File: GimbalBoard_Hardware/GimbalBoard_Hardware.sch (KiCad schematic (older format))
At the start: 5 parts

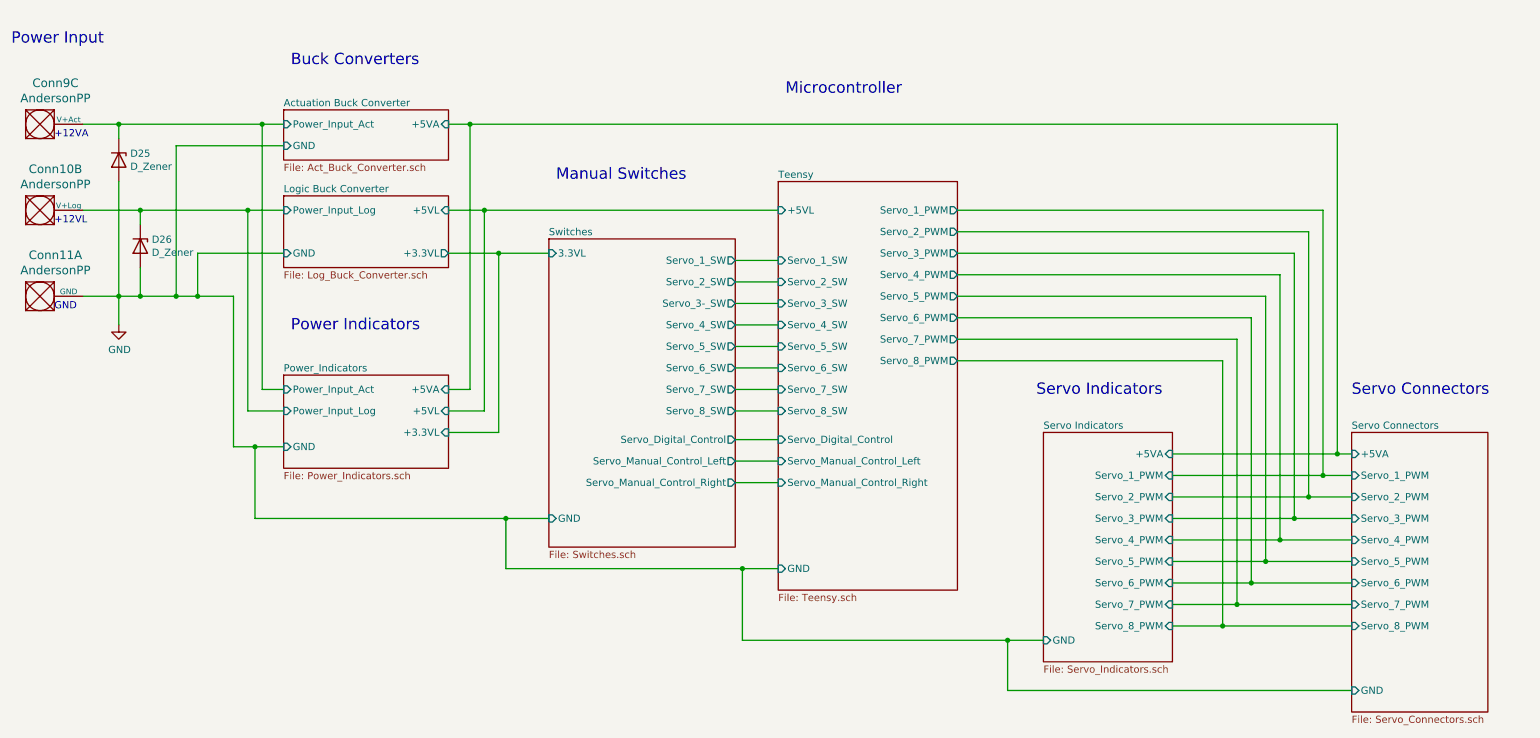
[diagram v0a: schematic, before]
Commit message: Post PDR changes
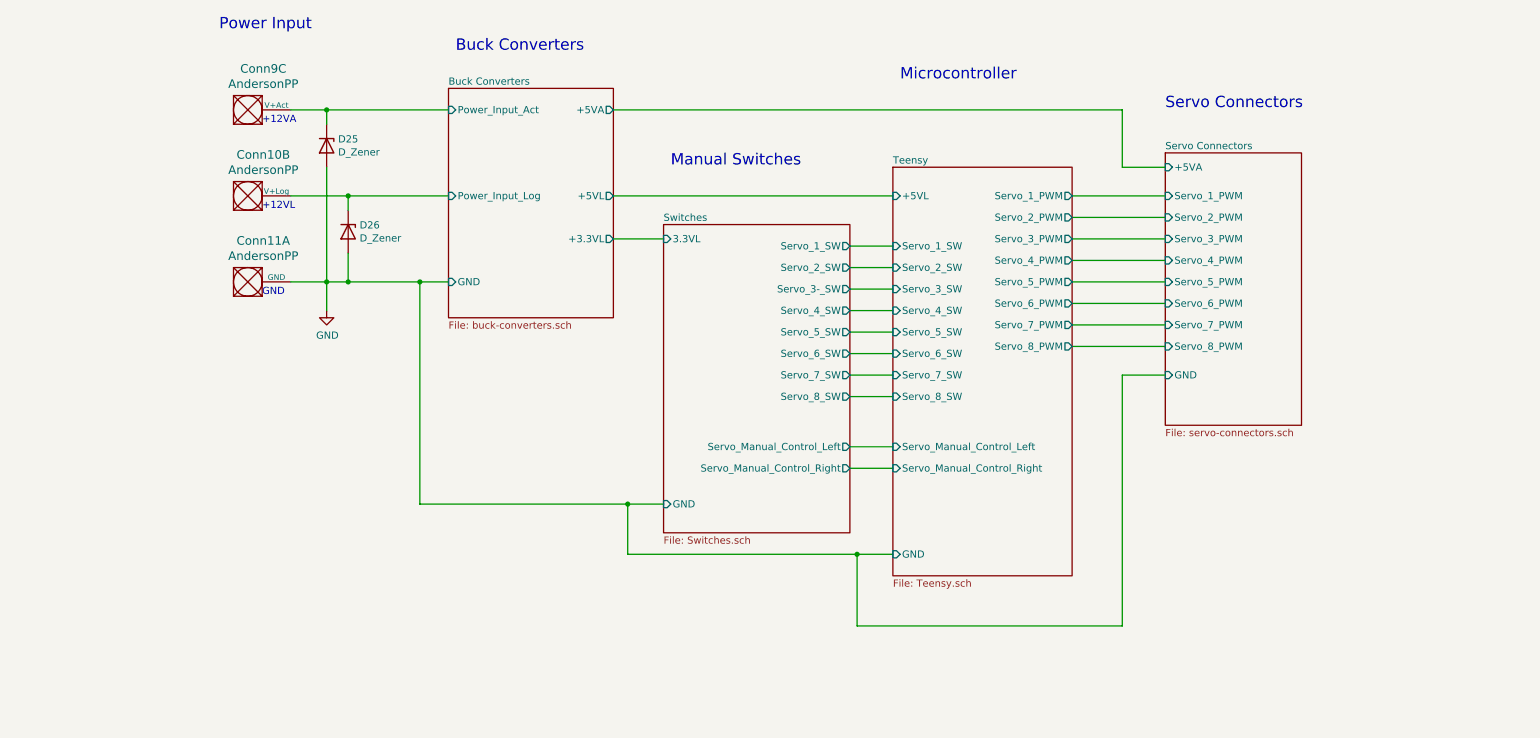
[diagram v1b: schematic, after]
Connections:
- net Actuation Buck Converter/Power_Input_Act renamed Buck Converters/Power_Input_Act
- net Logic Buck Converter/Power_Input_Log renamed Buck Converters/Power_Input_Log
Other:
- note added: "Servo Connectors"
- note removed: "Power Indicators"
- note removed: "Servo Connectors\n"
- note removed: "Servo Indicators"
- moved on the sheet: Conn10B, Conn11A, Conn9C, D25, D26
